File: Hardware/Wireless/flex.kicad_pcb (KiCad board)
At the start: 2 copper layers, 14.2 x 9.7 mm, 1 part

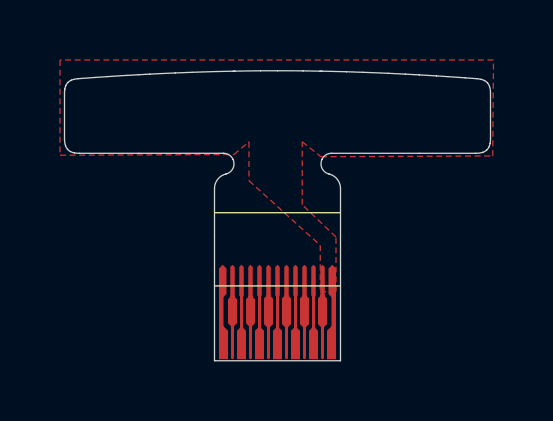
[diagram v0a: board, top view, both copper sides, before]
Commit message: current version
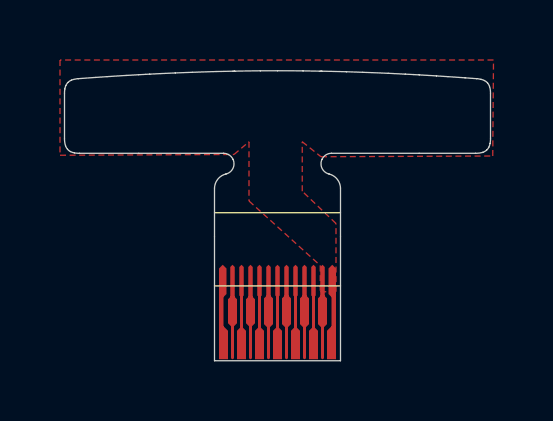
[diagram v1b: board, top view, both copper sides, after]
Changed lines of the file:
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@@
 		(48 "B.Fab" user)
 		(49 "F.Fab" user)
-		(50 "User.1" user)
+		(50 "User.1" user "PI stiffener")
 		(51 "User.2" user)
 		(52 "User.3" user)
@@
 			(layer "F.SilkS"
 				(type "Top Silk Screen")
+				(color "White")
 			)
 			(layer "F.Paste"
@@
 			(layer "F.Mask"
 				(type "Top Solder Mask")
-				(color "Black")
+				(color "Yellow")
 				(thickness 0.035)
 			)
@@
 			(layer "dielectric 1"
 				(type "core")
+				(color "Polyimide")
 				(thickness 0.012)
 				(material "FR4")
@@
 			(layer "B.Mask"
 				(type "Bottom Solder Mask")
-				(color "Black")
+				(color "Yellow")
 				(thickness 0.035)
 			)
@@
 			(layer "B.SilkS"
 				(type "Bottom Silk Screen")
+				(color "White")
 			)
 			(copper_finish "None")
@@
 		(allow_soldermask_bridges_in_footprints no)
 		(aux_axis_origin 171 95)
-		(grid_origin 171 95)
+		(grid_origin 168.9 95)
 		(pcbplotparams
-			(layerselection 0x00010fc_ffffffff)
+			(layerselection 0x00410fc_7fffffff)
 			(plot_on_all_layers_selection 0x0000000_00000000)
 			(disableapertmacros no)
@@
 			(drillshape 0)
 			(scaleselection 1)
-			(outputdirectory "../../../../../../../../Desktop/gerbers/wireless/")
+			(outputdirectory "../../../../../../../../Desktop/flex/")
 		)
 	)
@@
 		(layer "Edge.Cuts")
 	)
+	(gr_rect
+		(start 168.9 91.7)
+		(end 173.1 95)
+		(stroke
+			(width 0)
+			(type solid)
+		)
+		(fill solid)
+		(layer "User.1")
+	)
 	(gr_text "Tongtong.inc"
 		(at 174.449023 86.832953 0)
@@
 		(polygon
 			(pts
-				(xy 172.425 92.7) (xy 172.95 92.7) (xy 172.95 90.875) (xy 171.825 89.8) (xy 171.825 87.7) (xy 172.45 88.2)
+				(xy 172.425 92.7) (xy 172.95 92.7) (xy 172.95 90.425) (xy 171.825 89.35) (xy 171.825 87.7) (xy 172.45 88.2)
 				(xy 178.175 88.175) (xy 178.2 84.975) (xy 163.75 84.975) (xy 163.75 88.15) (xy 169.55 88.125) (xy 170.05 87.7)
-				(xy 170.05 89) (xy 172.425 91.15)
-			)
-		)
+				(xy 170.05 89.675) (xy 172.425 91.825)
+			)
+		)
